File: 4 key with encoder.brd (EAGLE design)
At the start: 105.2 x 42.9 mm, 24 parts, among them SW1 KEYSWITCH-PLAIN-MXHS-1U, SW2 KEYSWITCH-PLAIN-MXHS-1U, SW3 KEYSWITCH-PLAIN-MXHS-1U, SW4 KEYSWITCH-PLAIN-MXHS-1U, SW5 KEYSWITCH-PLAIN-MXHS-1U, SW6 KEYSWITCH-PLAIN-MXHS-1U

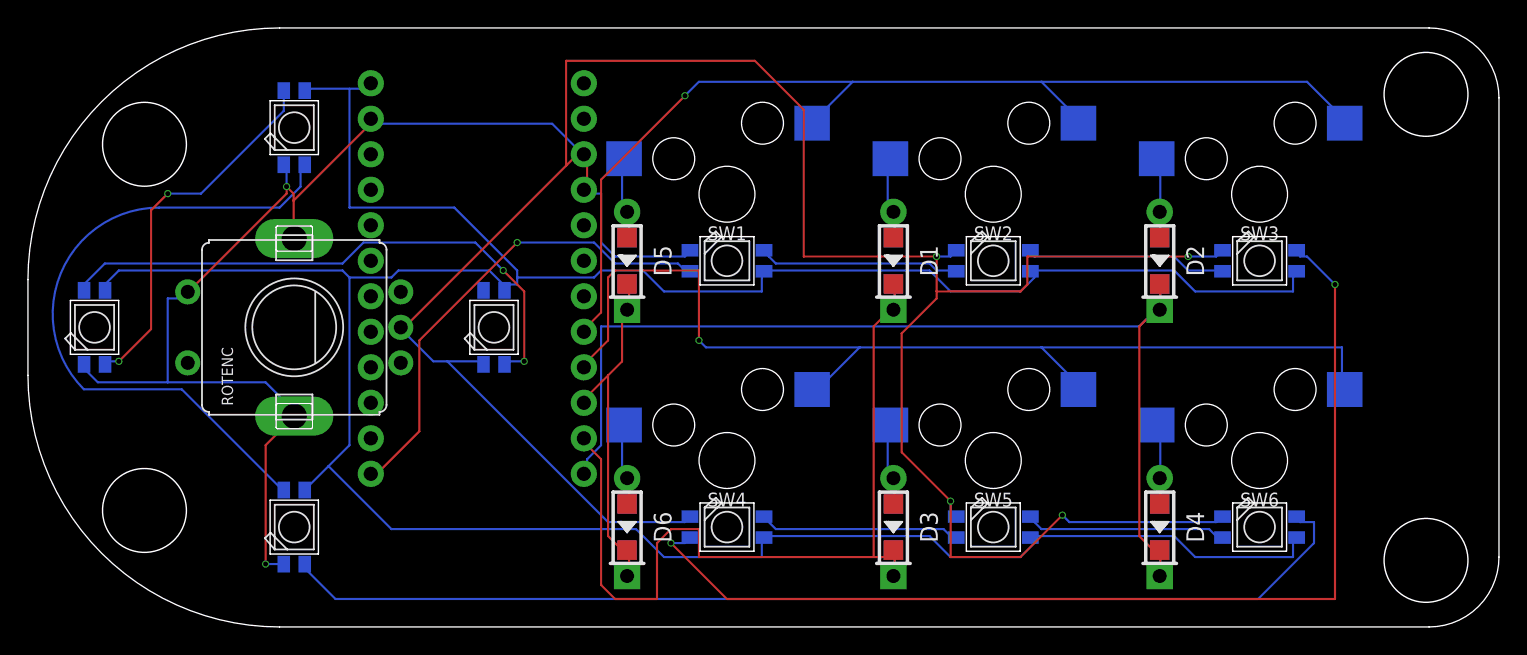
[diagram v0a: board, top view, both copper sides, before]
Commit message: tweaks
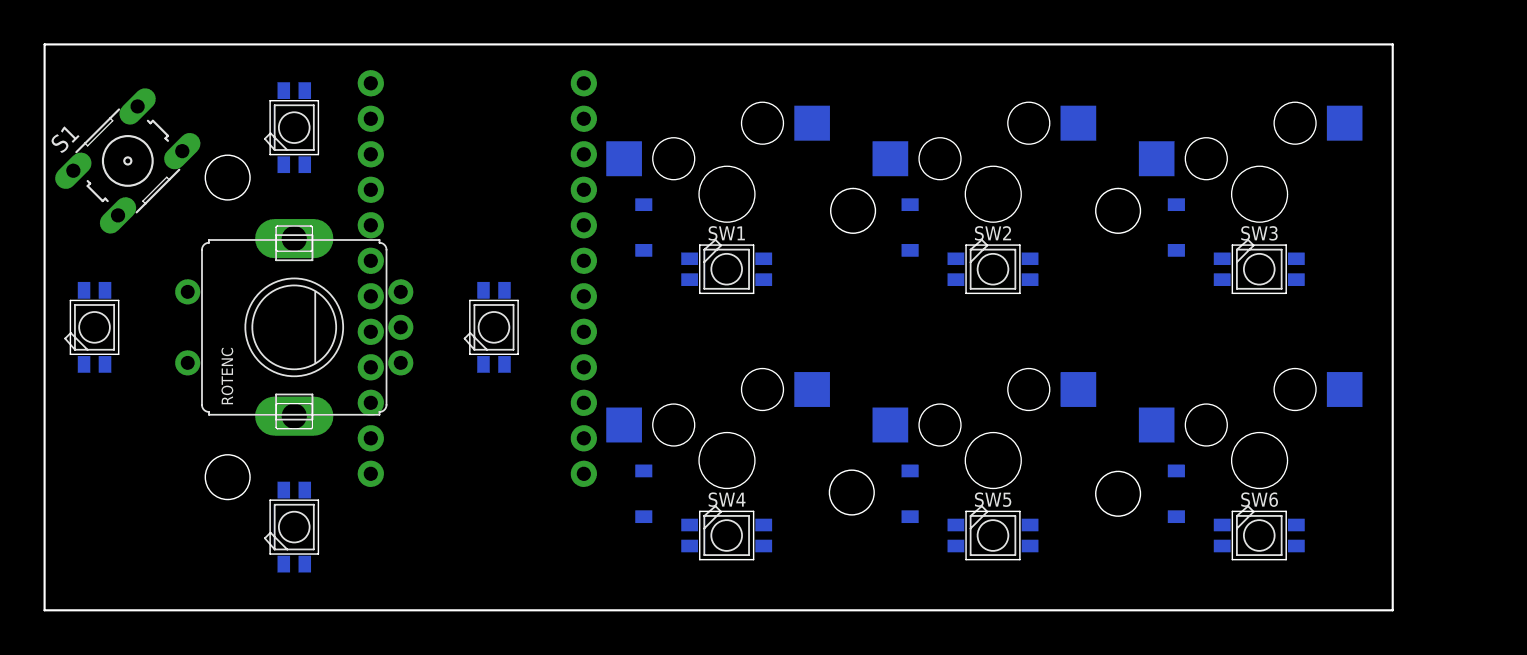
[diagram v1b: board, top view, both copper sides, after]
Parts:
- added S1: (no value), keeb-library:B3F-10XX
- B1: value SPARKFUN_PRO_MICRO -> (none)
- D1, D2, D3, D4, D5, D6: device keeb-library:DIODE_HAND -> keeb-library:SOD-123
- moved D6 2.66 mm to (44.1, 9.52), flipped to the bottom
- moved D5 2.66 mm to (44.1, 28.6), flipped to the bottom
- moved D3 2.66 mm to (63.1, 9.52), flipped to the bottom
- moved D1 2.66 mm to (63.1, 28.6), flipped to the bottom
- moved D4 2.66 mm to (82.2, 9.52), flipped to the bottom
- moved D2 2.66 mm to (82.2, 28.6), flipped to the bottom
- moved LED2 0.60 mm to (69.0, 25.6)
- moved LED5 0.60 mm to (69.0, 6.54)
- moved LED1 0.60 mm to (50.0, 25.6)
- moved LED4 0.60 mm to (50.0, 6.54)
- moved LED3 0.60 mm to (88.1, 25.6)
- moved LED6 0.60 mm to (88.1, 6.54)
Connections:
- new net RESET: B1.22, S1.1, S1.2
- net COL0: now also D5.C, D6.C; no longer D5.C1, D5.C2, D5.C3, D6.C1, D6.C2, D6.C3
- net COL1: now also D1.C, D3.C; no longer D1.C1, D1.C2, D1.C3, D3.C1, D3.C2, D3.C3
- net COL2: now also D2.C, D4.C; no longer D2.C1, D2.C2, D2.C3, D4.C1, D4.C2, D4.C3
- net GND: now also S1.3, S1.4
- net N$1: now also D5.A; no longer D5.A1, D5.A2, D5.A3
- net N$2: now also D6.A; no longer D6.A1, D6.A2, D6.A3
- net N$3: now also D3.A; no longer D3.A1, D3.A2, D3.A3
- net N$4: now also D1.A; no longer D1.A1, D1.A2, D1.A3
- net N$5: now also D2.A; no longer D2.A1, D2.A2, D2.A3
- net N$6: now also D4.A; no longer D4.A1, D4.A2, D4.A3
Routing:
- net GND: track 257.0 -> 0.00 mm, vias 6 -> 0
- net 5.0V: track 215.3 -> 0.00 mm
- net N$15: track 78.0 -> 0.00 mm
- net COL2: track 77.8 -> 0.00 mm
- net ROW1: track 77.5 -> 0.00 mm, vias 1 -> 0
- net N$12: track 77.0 -> 0.00 mm, vias 2 -> 0
- net ROW0: track 77.0 -> 0.00 mm, vias 1 -> 0
- net COL1: track 64.9 -> 0.00 mm
- net N$16: track 43.9 -> 0.00 mm
- net N$18: track 41.1 -> 0.00 mm, vias 2 -> 0
- net LED: track 34.3 -> 0.00 mm, vias 1 -> 0
- net COL0: track 29.0 -> 0.00 mm
- net N$17: track 26.9 -> 0.00 mm, vias 2 -> 0
- net N$11: track 14.4 -> 0.00 mm
- net N$8: track 14.4 -> 0.00 mm
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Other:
- board size 105.2 x 42.9 mm -> 96.4 x 40.5 mm
